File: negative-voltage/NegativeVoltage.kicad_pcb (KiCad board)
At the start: 2 copper layers, 53.3 x 69.9 mm, 11 parts, among them J1 Screw_Terminal_01x02, J2 Screw_Terminal_01x02, U1 LM555

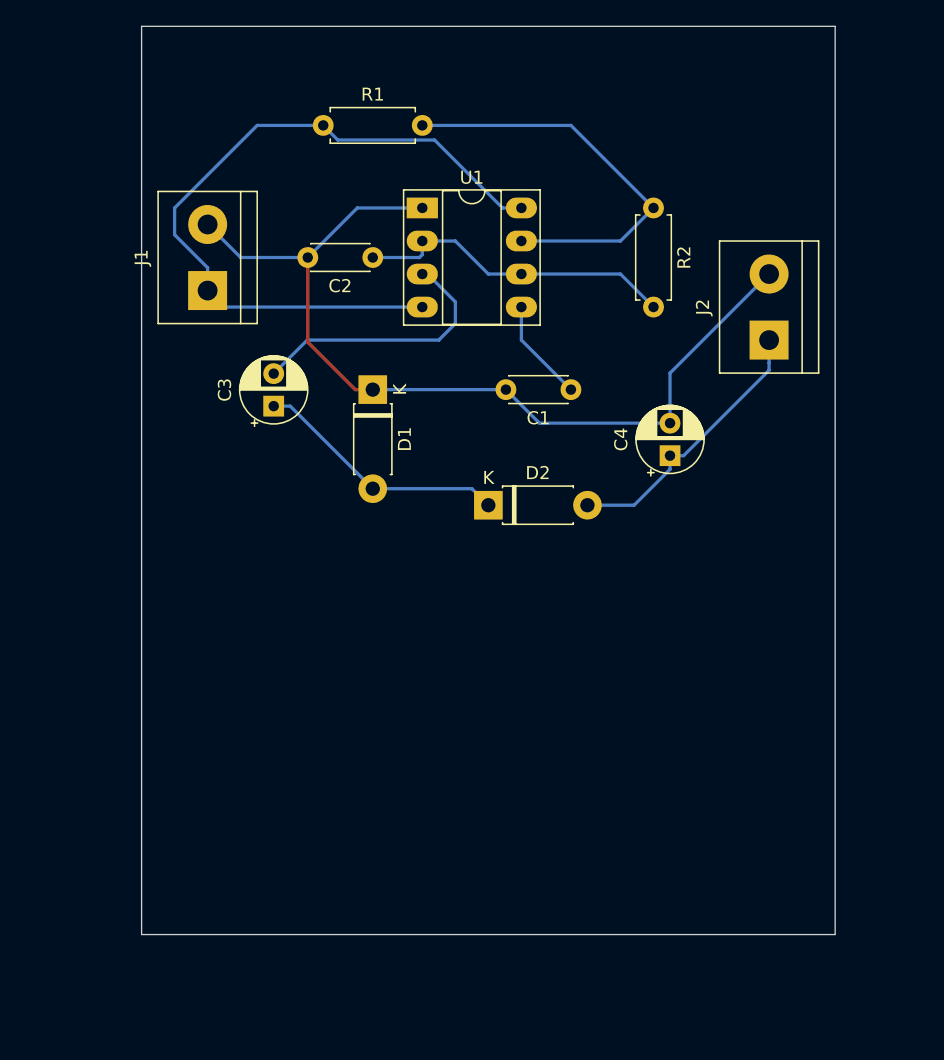
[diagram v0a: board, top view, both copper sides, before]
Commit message: Moves some stuff around
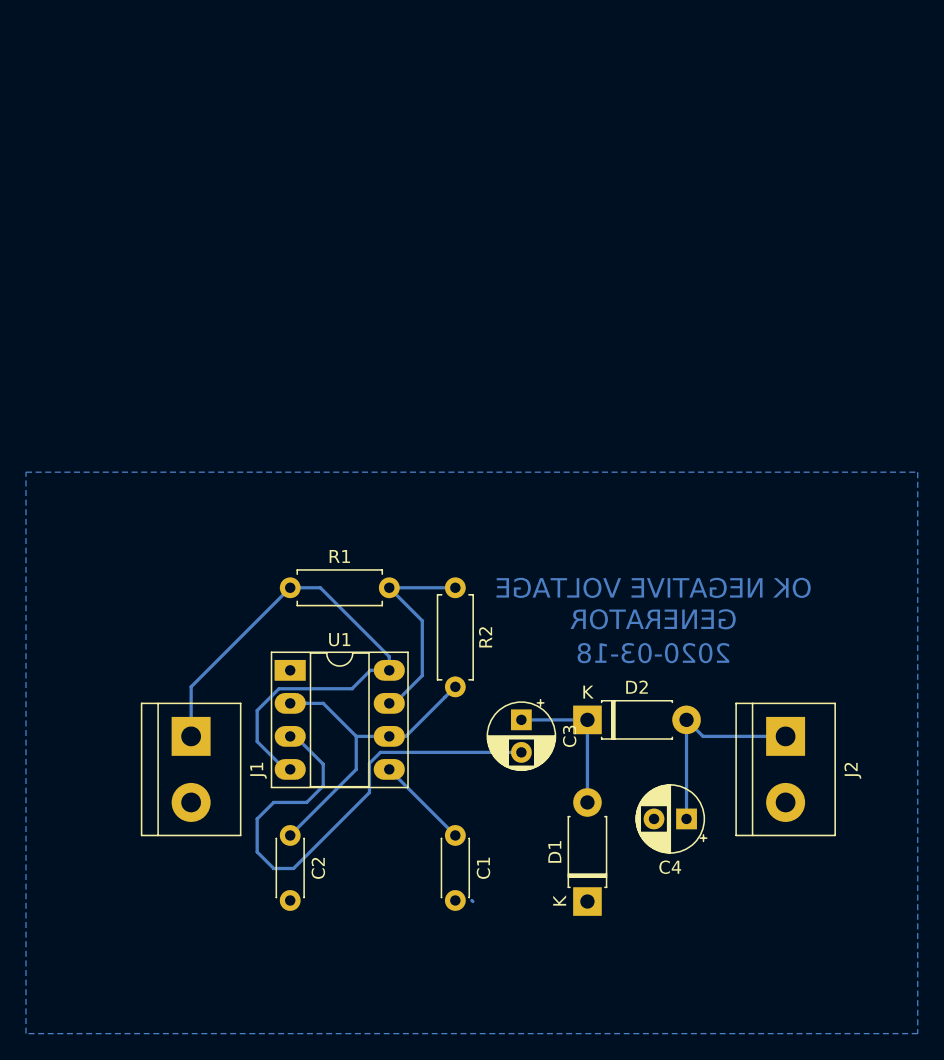
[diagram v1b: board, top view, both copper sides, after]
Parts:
- moved C2 44.9 mm to (62.2, 154.9), turned to 270 degrees
- moved D1 42.7 mm to (85.1, 160.0), turned to 90 degrees
- moved U1 37.0 mm to (62.2, 142.2)
- moved R1 35.7 mm to (62.2, 135.9)
- moved C1 35.4 mm to (74.9, 154.9), turned to 270 degrees
- moved J1 34.3 mm to (54.6, 147.3), turned to 270 degrees
- moved R2 32.9 mm to (74.9, 135.9)
- moved C3 30.7 mm to (80.0, 146.1), turned to 270 degrees
- moved J2 30.5 mm to (100.3, 147.3), turned to 270 degrees
- moved C4 28.0 mm to (92.7, 153.7), turned to 180 degrees
- moved D2 18.2 mm to (85.1, 146.1)
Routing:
- net GND: track 70.7 -> 0.59 mm
- net N$4: track 20.7 -> 39.6 mm
- net N$3: track 31.6 -> 16.3 mm
- net VCC: track 56.4 -> 42.7 mm
- net N$5: track 19.7 -> 11.4 mm
- net N$6: track 21.2 -> 15.8 mm
- net N$1: track 24.8 -> 26.7 mm
- net N$2: track 7.93 -> 7.18 mm
- added copper zone on B.Cu, net GND
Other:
- board outline removed
- board text added: "2020-03-18"
- board text added: "OK NEGATIVE VOLTAGE GENERATOR"

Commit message: Increase solder mask clearance
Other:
- rule pad_to_mask_clearance: 0.051 -> 0.2
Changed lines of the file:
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@@
     (pad_size 1.524 1.524)
     (pad_drill 0.762)
-    (pad_to_mask_clearance 0.051)
+    (pad_to_mask_clearance 0.2)
     (solder_mask_min_width 0.25)
     (aux_axis_origin 0 0)
     (visible_elements 7FFFFFFF)
     (pcbplotparams
-      (layerselection 0x010fc_ffffffff)
+      (layerselection 0x00040_fffffffe)
       (usegerberextensions false)
       (usegerberattributes false)
@@
       (padsonsilk false)
       (subtractmaskfromsilk false)
-      (outputformat 1)
+      (outputformat 5)
       (mirror false)
       (drillshape 1)

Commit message: Make a subcircuit for the pwm generator
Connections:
- C3 pad 2: N$4 (its old number) -> PWM_SIGNAL
- U1 pad 3: N$4 (its old number) -> PWM_SIGNAL
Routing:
- net PWM_SIGNAL: track 0.00 -> 39.6 mm
- net N$4 (its old number): track 39.6 -> 0.00 mm
